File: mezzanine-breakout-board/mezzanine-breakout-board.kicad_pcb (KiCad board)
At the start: 2 copper layers, 19.5 x 30 mm, 2 parts, among them J1 Mezzanine Plug, J2 Conn_01x10

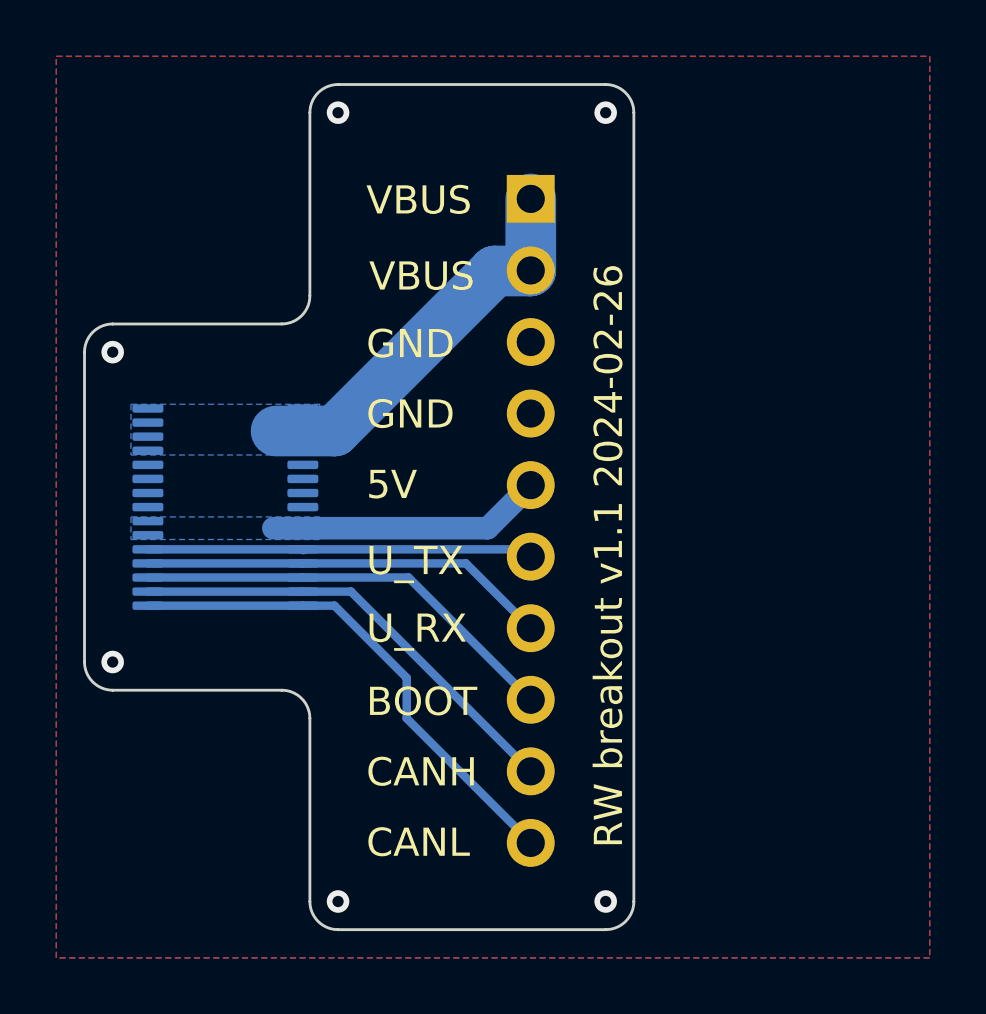
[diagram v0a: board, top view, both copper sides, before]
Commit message: version, date, and possibly other changes and switched to v8
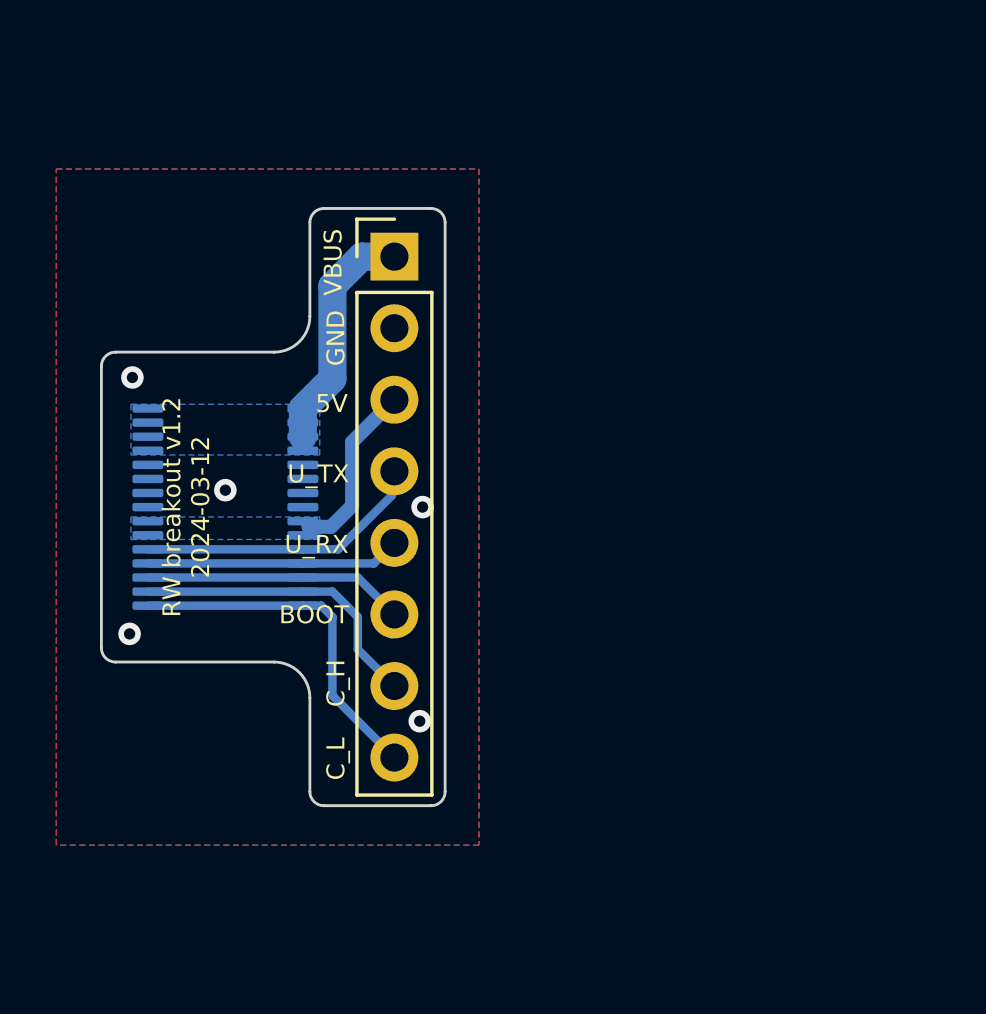
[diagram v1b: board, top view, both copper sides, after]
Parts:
- J2: footprint Connector_PinHeader_2.54mm:PinHeader_1x10_P2.54mm_Vertical -> Connector_PinHeader_2.54mm:PinHeader_1x08_P2.54mm_Vertical; moved to F.Cu
- moved J2 5.26 mm to (128.0, 97.1), turned to 0 degrees
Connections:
- J2 pad 2: /VBUS -> /GND
- J2 pad 3: /GND -> /5V
- J2 pad 4: /GND -> /UART_TX
- J2 pad 5: /5V -> /UART_RX
- J2 pad 6: /UART_TX -> /BOOT
- J2 pad 7: /UART_RX -> /CAN_H
- J2 pad 8: /BOOT -> /CAN_L
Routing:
- net /CAN_H: track 16.2 -> 10.7 mm
- net /VBUS: track 13.9 -> 8.42 mm
- net /UART_RX: track 14.5 -> 9.05 mm
- net /BOOT: track 15.4 -> 9.97 mm
- net /CAN_L: track 17.9 -> 12.6 mm
- net /UART_TX: track 13.8 -> 9.59 mm
- net /5V: track 9.77 -> 6.52 mm
- net /GND: vias 6 -> 5
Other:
- board size 19.5 x 30 mm -> 12.2 x 21.2 mm
- board text added: "C_H"
- board text added: "C_L"
- board text added: "RW breakout v1.2 2024-03-12"
- board text removed: "CANH"
- board text removed: "CANL"
- board text removed: "RW breakout v1.1 2024-02-26"
